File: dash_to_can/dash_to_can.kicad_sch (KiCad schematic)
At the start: 64 parts, among them J1 AVR-ISP1, J2 Conn_02x10_Top_Bottom, Q1 2N3904, Q10 AO3401A, Q2 2N3904, Q3 2N3904, Q4 AO3401A, Q5 2N3904, Q6 AO3401A, Q7 2N3904, Q8 AO3401A, Q9 2N3904, U1 ATmega328P-A, U2 LM2575-5.0BU, U3 MCP2515-xST, U4 TJA1050T_CM_118, U5 ULN2003A, U6 MCP41010, Y1 20MHz, Y2 16MHz

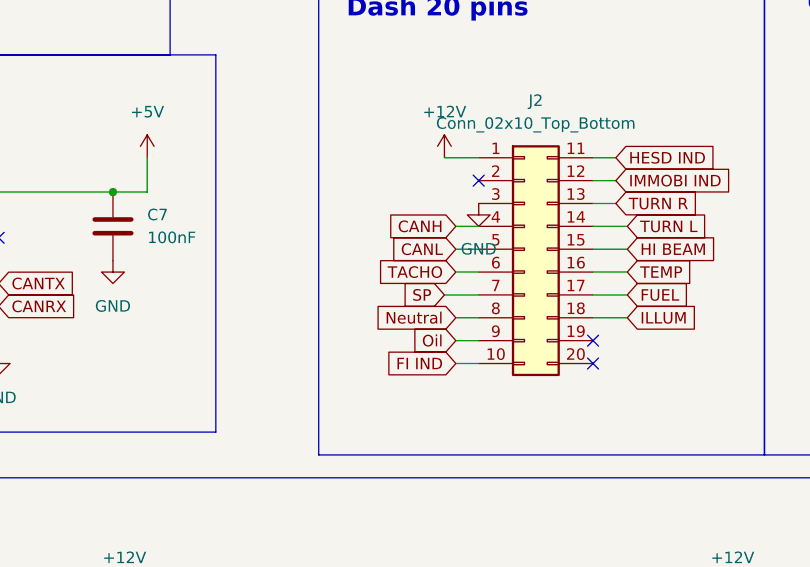
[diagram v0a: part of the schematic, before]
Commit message: 2nd draft (with stuff I didn't save)
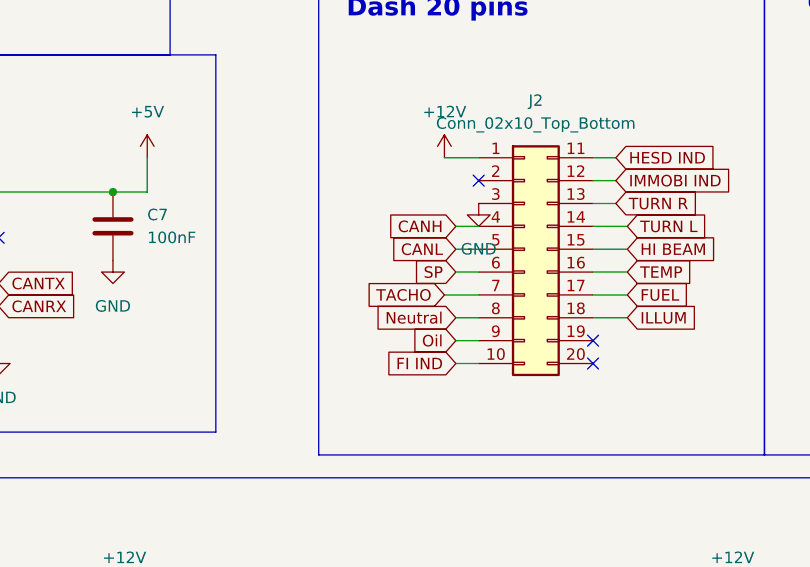
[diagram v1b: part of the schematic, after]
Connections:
- net SP: now also J2.6 (Pin_6); no longer J2.7 (Pin_7)
- net TACHO: now also J2.7 (Pin_7); no longer J2.6 (Pin_6)
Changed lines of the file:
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@@
 		)
 	)
-	(global_label "SP"
+	(global_label "TACHO"
 		(shape input)
 		(at 119.38 102.87 180)
@@
 		)
 		(property "Intersheetrefs" "${INTERSHEET_REFS}"
-			(at 113.9153 102.87 0)
+			(at 110.4076 102.87 0)
 			(effects
 				(font
@@
 		)
 	)
-	(global_label "TACHO"
+	(global_label "SP"
 		(shape input)
 		(at 120.65 100.33 180)
@@
 		)
 		(property "Intersheetrefs" "${INTERSHEET_REFS}"
-			(at 111.6776 100.33 0)
+			(at 115.1853 100.33 0)
 			(effects
 				(font
